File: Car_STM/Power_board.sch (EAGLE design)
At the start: 36 parts, among them K1 S22, K10 G2RE, K11 G2RE, K2 G2RE, K3 S22, K4 S22, K5 S22, K6 S22, K7 S22, K8 HY1-12V, K9 HY1-12V, Q2 IRFR5305, X11 1751251, X13 1751248, X9 1751251

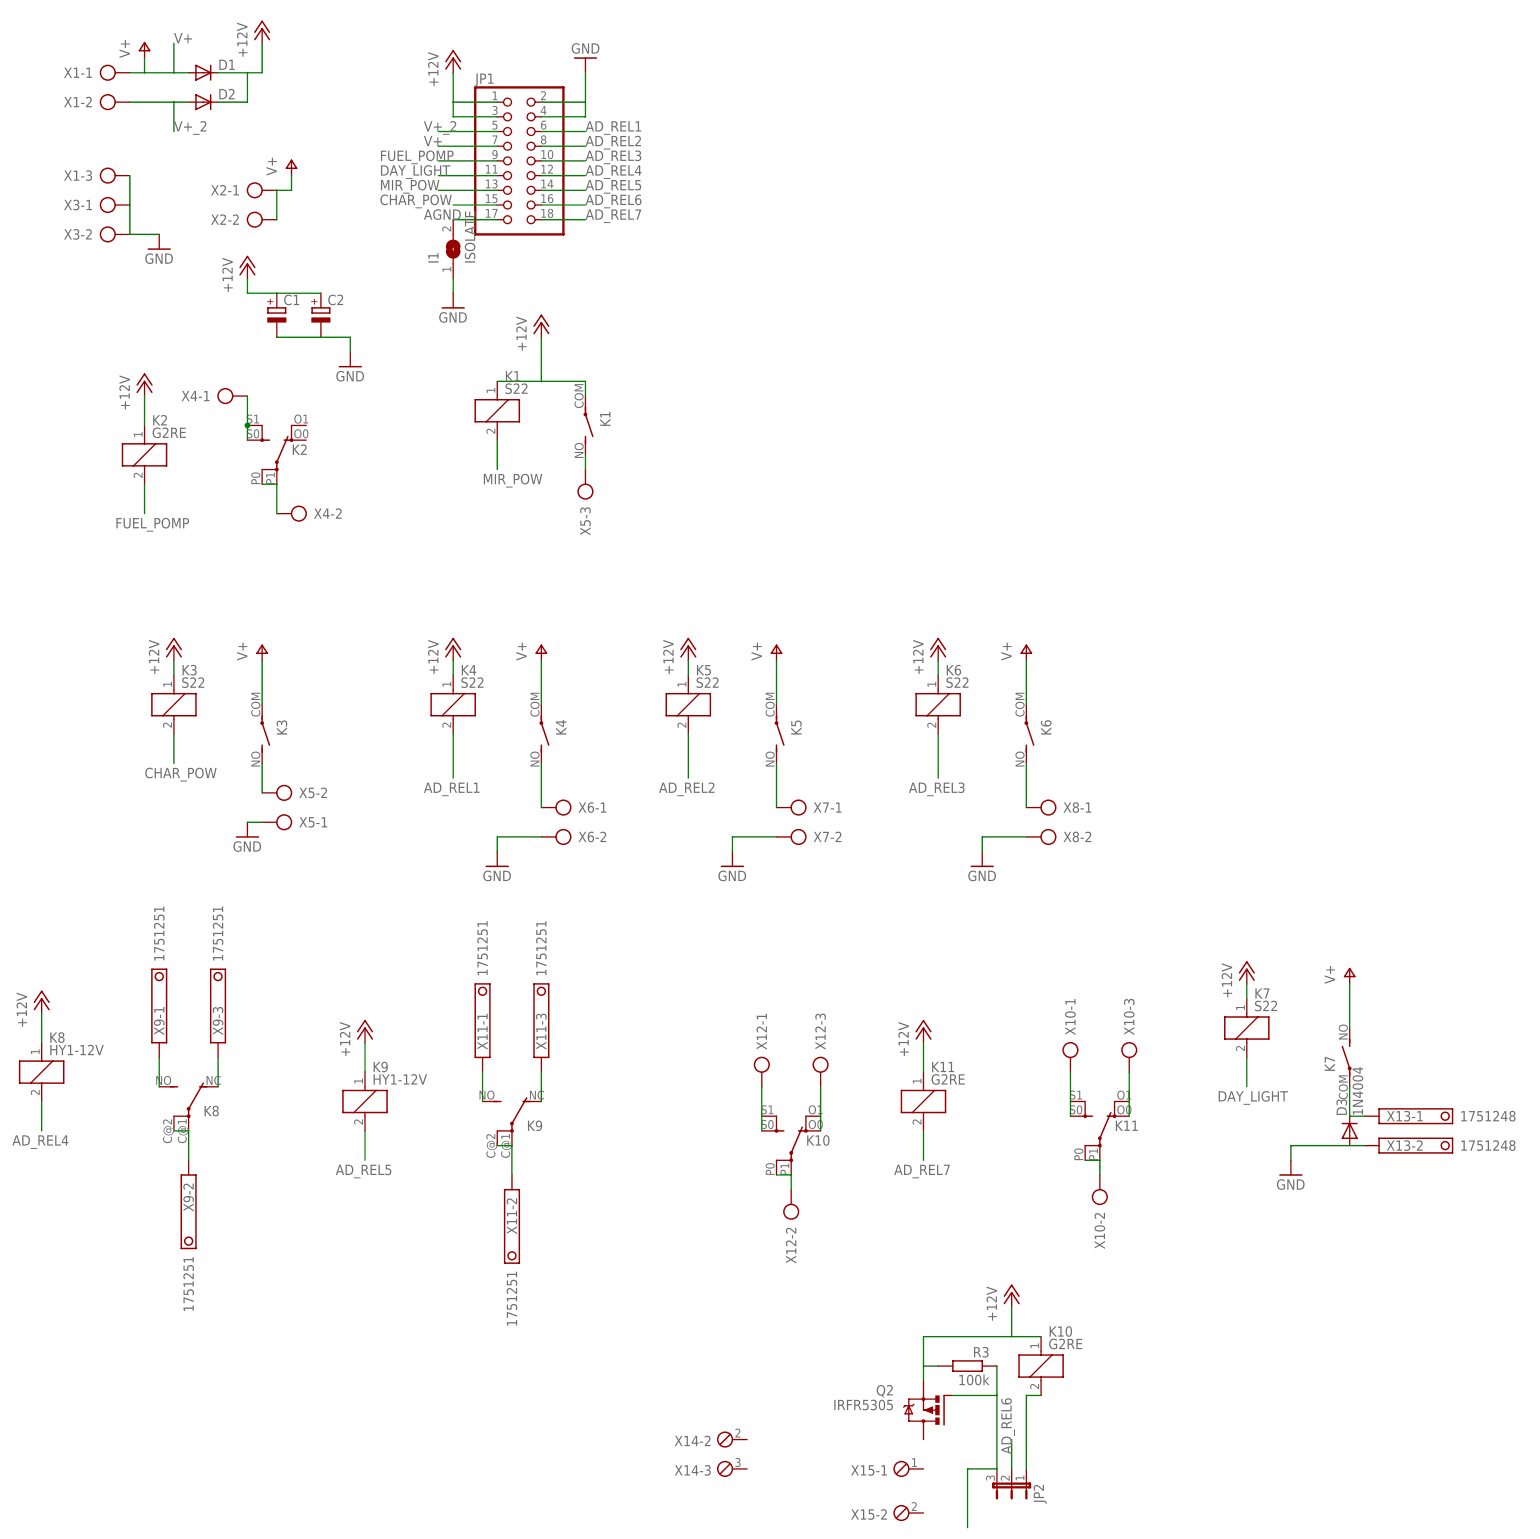
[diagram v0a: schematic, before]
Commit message: V1.25 Just tittle missing
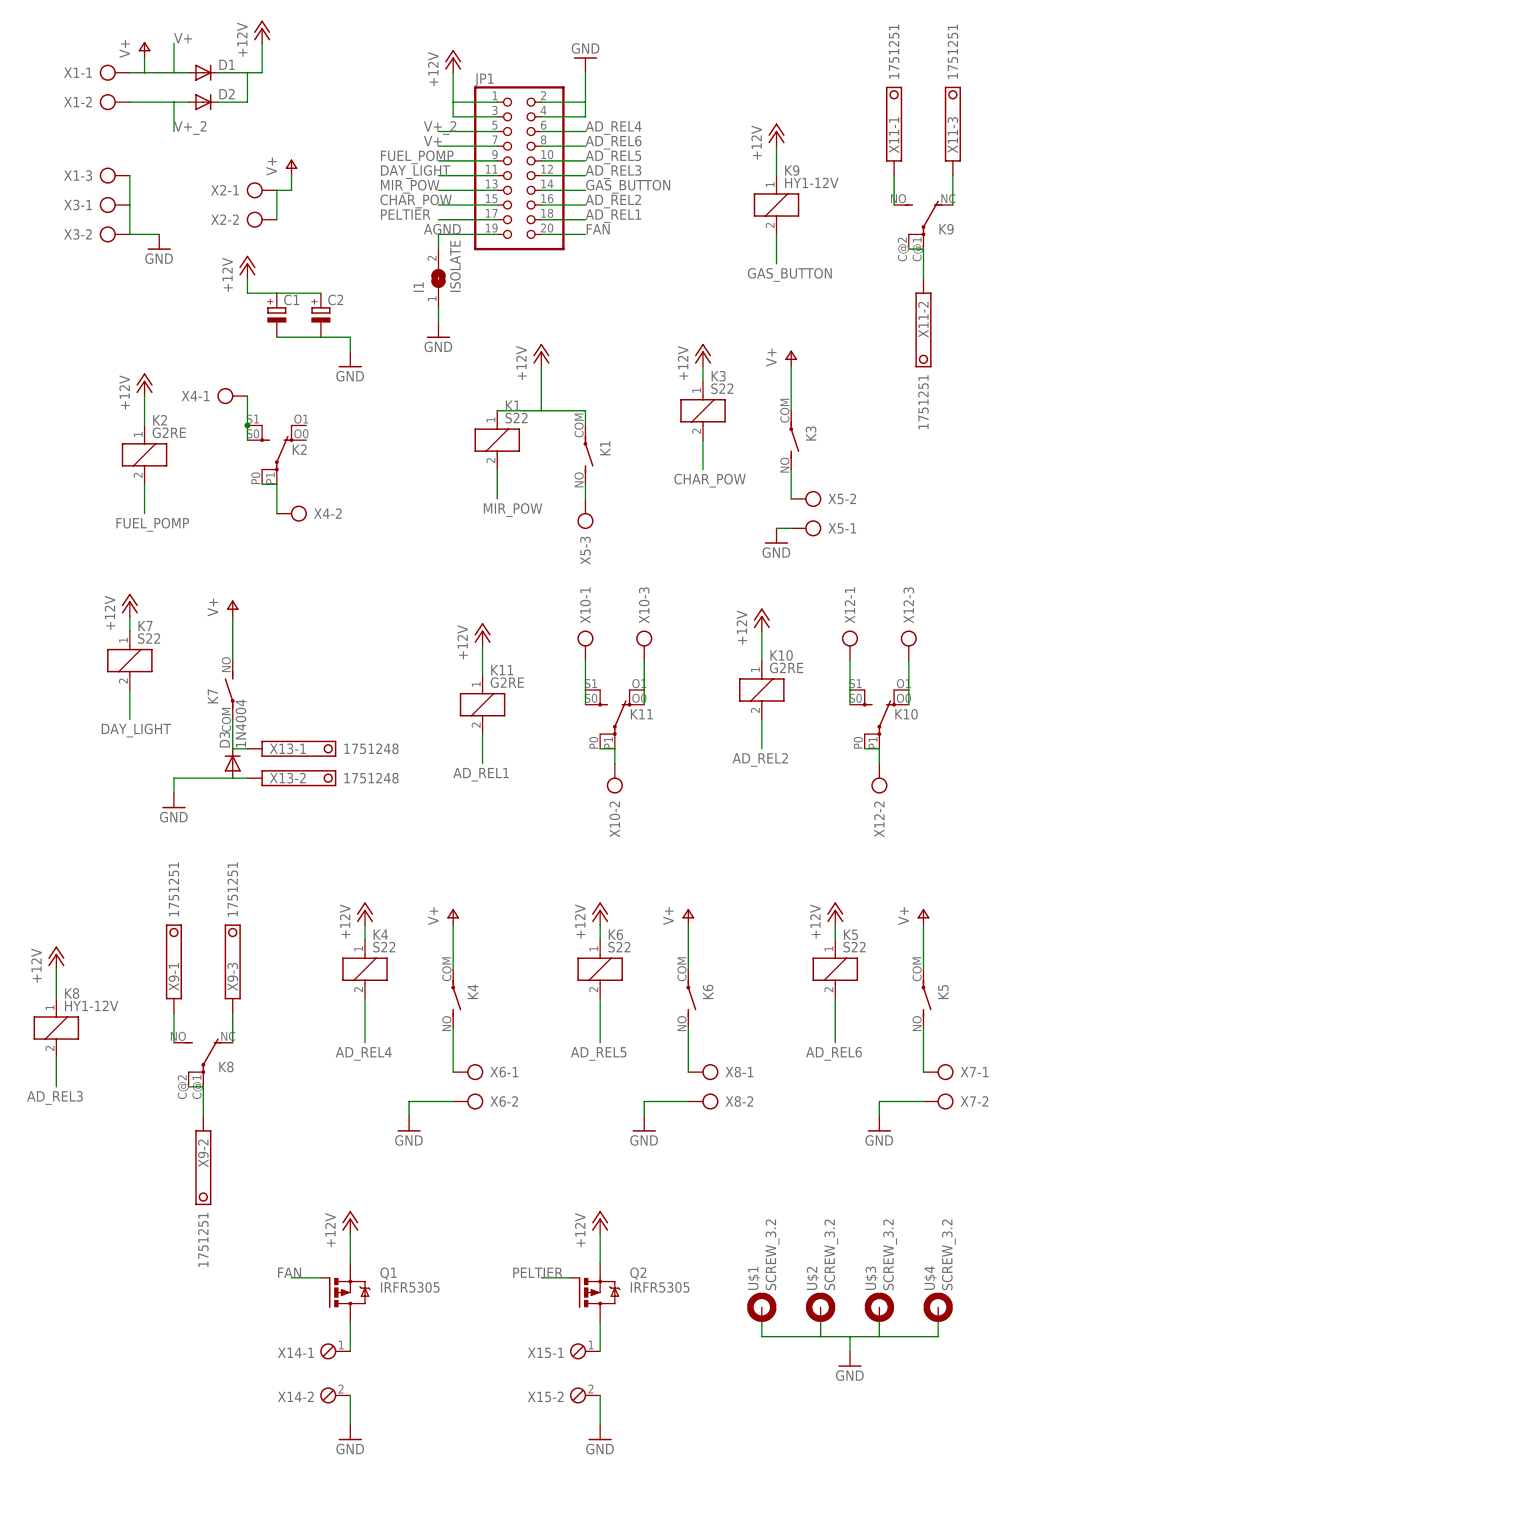
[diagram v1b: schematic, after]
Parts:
- removed JP2: (no value), jumper:JP2E
- removed R3: 100k, resistor:R-EU_R0805
- added Q1: IRFR5305, transistor-power:IRFR5305
- added U$1, U$2, U$3, U$4: SCREW_3.2, Stworzone:SCREW_3.2
- JP1: device pinhead:PINHD-2X9 -> pinhead:PINHD-2X10
- X14: device con-phoenix-254:MPT3 -> con-phoenix-254:MPT2
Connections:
- removed net AD_REL7: JP1.18, K111.2
- removed net N$44: JP2.3, Q2.G, R3.1
- removed net N$7: JP2.1, K101.2
- new net FAN: JP1.20, Q1.G
- new net GAS_BUTTON: JP1.14, K91.2
- new net N$6: Q1.D, X14-1.1
- new net N$9: Q2.D, X15-1.1
- new net PELTIER: JP1.17, Q2.G
- net +12V: now also Q1.S; no longer R3.2
- net AD_REL1: now also JP1.18, K111.2; no longer JP1.6, K4G$2.2
- net AD_REL2: now also JP1.16, K101.2; no longer JP1.8, K5G$2.2
- net AD_REL3: now also JP1.12, K81.2; no longer JP1.10, K6G$2.2
- net AD_REL4: now also JP1.6, K4G$2.2; no longer JP1.12, K81.2
- net AD_REL5: now also JP1.10, K6G$2.2; no longer JP1.14, K91.2
- net AD_REL6: now also JP1.8, K5G$2.2; no longer JP1.16, JP2.2
- net AGND: now also JP1.19; no longer JP1.17
- net GND: now also U$1.MOUNT, U$2.MOUNT, U$3.MOUNT, U$4.MOUNT, X14-2.1, X15-2.1
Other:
- moved on the sheet: D3, I1, K1, K10, K11, K3, K4, K5, K6, K7, K8, K9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
